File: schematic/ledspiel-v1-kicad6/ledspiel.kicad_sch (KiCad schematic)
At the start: 133 parts, among them J1 Conn_Battery, J3 USART Debug, J4 Micro_SD_Card, J5 USB_B_Micro, J50 Conn_01x16_Male, Q1 BSS138, Q10 BSS138, Q11 BSS138, Q12 BSS138, Q13 BSS138, Q14 BSS138, Q40 IRLML6402, Q60 SFH300-3/4, U1 STM32F405RGTx, U2 USBLC6-2SC6, U3 MCP1640CH, U4 LP38693MP-3.3, U6 TSOP312xx, Y1 8MHz, Y2 32768Hz

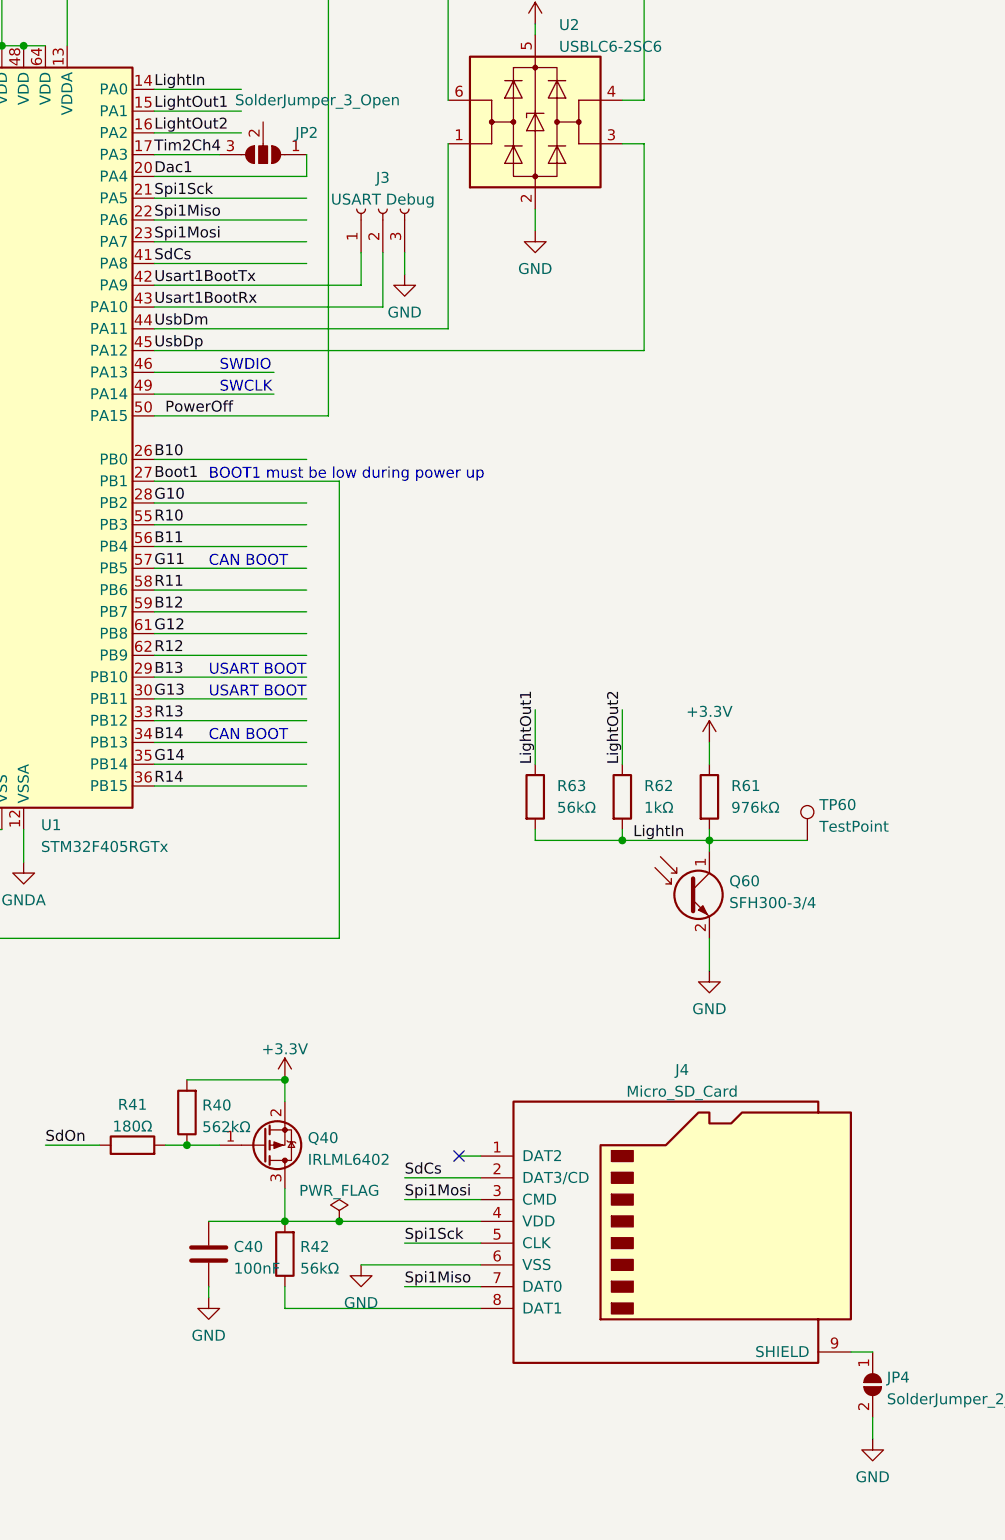
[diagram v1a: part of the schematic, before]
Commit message: WIP: Add LM
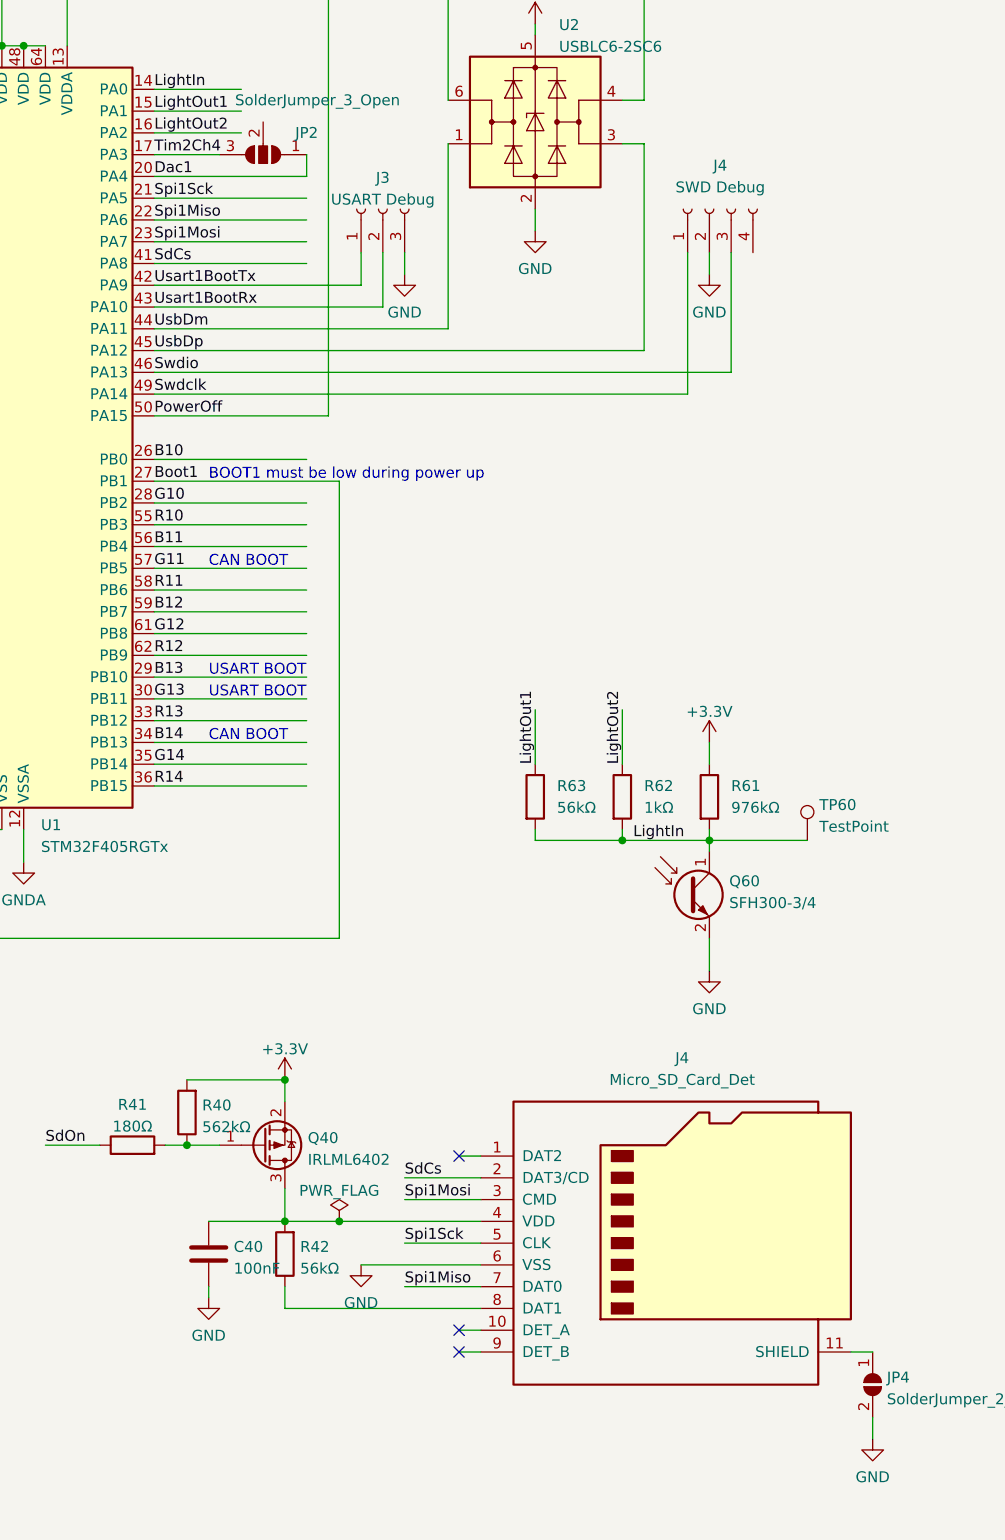
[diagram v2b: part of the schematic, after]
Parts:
- removed J4: Micro_SD_Card, symbol Connector:Micro_SD_Card
- added J4: SWD Debug, symbol Connector:Conn_01x04_Female
- added J4: Micro_SD_Card_Det, symbol Connector:Micro_SD_Card_Det
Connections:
- net GND: now also J4.2 (Pin_2), J4.6 (VSS)
- net SdCs: now also J4.2 (DAT3/CD)
- net Spi1Miso: now also J4.7 (DAT0)
- net Spi1Mosi: now also J4.3 (CMD)
- net Spi1Sck: now also J4.5 (CLK)
- net Swdio: now reaches U1.46 (PA13)
- net Swdio: now also J4.3 (Pin_3)
- net Swdclk: now reaches U1.49 (PA14)
- net Swdclk: now also J4.1 (Pin_1)
- net at R42.1: now also J4.8 (DAT1)
- net at C40.1, Q40.3 (D), R42.2: now also J4.4 (VDD)
- net at JP4.1 (A): now also J4.11 (SHIELD)
- no-connect marks 2 -> 4
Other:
- note removed: "SWCLK"
- note removed: "SWDIO"
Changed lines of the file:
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@@
   (junction (at 67.31 55.88) (diameter 0) (color 0 0 0 0)
   )
+  (no_connect (at 157.48 250.19))
   (no_connect (at 173.99 78.74))
   (no_connect (at 157.48 229.87))
+  (no_connect (at 157.48 252.73))
   (wire (pts (xy 299.72 77.47) (xy 299.72 102.87))
     (stroke (width 0) (type default) (color 0 0 0 0))
@@
     (stroke (width 0) (type default) (color 0 0 0 0))
   )
-  (wire (pts (xy 121.92 138.43) (xy 135.89 138.43))
+  (wire (pts (xy 121.92 138.43) (xy 189.23 138.43))
     (stroke (width 0) (type default) (color 0 0 0 0))
   )
@@
     (stroke (width 0) (type default) (color 0 0 0 0))
   )
+  (wire (pts (xy 189.23 124.46) (xy 189.23 138.43))
+    (stroke (width 0) (type default) (color 0 0 0 0))
+  )
   (wire (pts (xy 297.18 107.95) (xy 297.18 133.35))
     (stroke (width 0) (type default) (color 0 0 0 0))
@@
     (stroke (width 0) (type default) (color 0 0 0 0))
   )
+  (wire (pts (xy 184.15 124.46) (xy 184.15 140.97))
+    (stroke (width 0) (type default) (color 0 0 0 0))
+  )
   (wire (pts (xy 121.92 184.15) (xy 139.7 184.15))
     (stroke (width 0) (type default) (color 0 0 0 0))
@@
     (stroke (width 0) (type default) (color 0 0 0 0))
   )
+  (wire (pts (xy 186.69 124.46) (xy 186.69 127))
+    (stroke (width 0) (type default) (color 0 0 0 0))
+  )
   (wire (pts (xy 67.31 44.45) (xy 67.31 45.72))
     (stroke (width 0) (type default) (color 0 0 0 0))
@@
     (stroke (width 0) (type default) (color 0 0 0 0))
   )
-  (wire (pts (xy 121.92 140.97) (xy 135.89 140.97))
+  (wire (pts (xy 121.92 140.97) (xy 184.15 140.97))
     (stroke (width 0) (type default) (color 0 0 0 0))
   )
@@
     (stroke (width 0) (type default) (color 0 0 0 0))
   )
+  (wire (pts (xy 157.48 252.73) (xy 160.02 252.73))
+    (stroke (width 0) (type default) (color 0 0 0 0))
+  )
   (wire (pts (xy 290.83 52.07) (xy 299.72 52.07))
     (stroke (width 0) (type default) (color 0 0 0 0))
@@
     (stroke (width 0) (type default) (color 0 0 0 0))
   )
+  (wire (pts (xy 157.48 250.19) (xy 160.02 250.19))
+    (stroke (width 0) (type default) (color 0 0 0 0))
+  )
   (wire (pts (xy 151.13 86.36) (xy 151.13 83.82))
     (stroke (width 0) (type default) (color 0 0 0 0))
@@
     (effects (font (size 1.27 1.27)) (justify left bottom))
   )
-  (text "SWCLK" (at 129.54 140.97 0)
-    (effects (font (size 1.27 1.27)) (justify left bottom))
-  )
-  (text "SWDIO" (at 129.54 138.43 0)
-    (effects (font (size 1.27 1.27)) (justify left bottom))
-  )
   (label "Line5" (at 241.3 149.86 0)
     (effects (font (size 1.27 1.27)) (justify left bottom))
@@
     (effects (font (size 1.27 1.27)) (justify left bottom))
   )
+  (label "Swdio" (at 121.92 138.43 0)
+    (effects (font (size 1.27 1.27)) (justify left bottom))
+  )
+  (label "Swdclk" (at 121.92 140.97 0)
+    (effects (font (size 1.27 1.27)) (justify left bottom))
+  )
   (label "Line5" (at 81.28 158.75 0)
     (effects (font (size 1.27 1.27)) (justify left bottom))
@@
     (effects (font (size 1.27 1.27)) (justify left bottom))
   )
-  (label "PowerOff" (at 123.19 143.51 0)
+  (label "PowerOff" (at 121.92 143.51 0)
     (effects (font (size 1.27 1.27)) (justify left bottom))
   )
@@
     (pin "1")
   )
+  (symbol (lib_id "Connector:Conn_01x04_Female") (at 186.69 119.38 90) (unit 1)
+    (in_bom yes) (on_board yes) (fields_autoplaced)
+    (property "Reference" "J4" (id 0) (at 187.96 114.3 90))
+    (property "Value" "SWD Debug" (id 1) (at 187.96 116.84 90))
+    (property "Footprint" "" (id 2) (at 186.69 119.38 0)
+      (effects (font (size 1.27 1.27)) hide)
+    )
+    (property "Datasheet" "~" (id 3) (at 186.69 119.38 0)
+      (effects (font (size 1.27 1.27)) hide)
+    )
+    (pin "1")
+    (pin "2")
+    (pin "3")
+    (pin "4")
+  )
   (symbol (lib_id "power:GND") (at 146.05 242.57 0) (unit 1)
     (in_bom yes) (on_board yes) (fields_autoplaced)
@@
     (pin "3")
   )
-  (symbol (lib_id "Connector:Micro_SD_Card") (at 182.88 237.49 0) (unit 1)
-    (in_bom yes) (on_board yes) (fields_autoplaced)
-    (property "Reference" "J4" (id 0) (at 183.515 219.8202 0))
-    (property "Value" "Micro_SD_Card" (id 1) (at 183.515 222.3571 0))
-    (property "Footprint" "" (id 2) (at 212.09 229.87 0)
-      (effects (font (size 1.27 1.27)) hide)
-    )
-    (property "Datasheet" "http://katalog.we-online.de/em/datasheet/693072010801.pdf" (id 3) (at 182.88 237.49 0)
-      (effects (font (size 1.27 1.27)) hide)
-    )
-    (pin "1")
-    (pin "2")
-    (pin "3")
-    (pin "4")
-    (pin "5")
-    (pin "6")
-    (pin "7")
-    (pin "8")
-    (pin "9")
-  )
   (symbol (lib_id "Device:LED_RKGB") (at 285.75 133.35 0) (unit 1)
     (in_bom yes) (on_board yes) (fields_autoplaced)
@@
     (pin "1")
   )
+  (symbol (lib_id "Connector:Micro_SD_Card_Det") (at 182.88 240.03 0) (unit 1)
+    (in_bom yes) (on_board yes) (fields_autoplaced)
+    (property "Reference" "J4" (id 0) (at 183.515 218.44 0))
+    (property "Value" "Micro_SD_Card_Det" (id 1) (at 183.515 220.98 0))
+    (property "Footprint" "" (id 2) (at 234.95 222.25 0)
+      (effects (font (size 1.27 1.27)) hide)
+    )
+    (property "Datasheet" "https://www.hirose.com/product/en/download_file/key_name/DM3/category/Catalog/doc_file_id/49662/?file_category_id=4&item_id=195&is_series=1" (id 3) (at 182.88 237.49 0)
+      (effects (font (size 1.27 1.27)) hide)
+    )
+    (pin "1")
+    (pin "10")
+    (pin "11")
+    (pin "2")
+    (pin "3")
+    (pin "4")
+    (pin "5")
+    (pin "6")
+    (pin "7")
+    (pin "8")
+    (pin "9")
+  )
   (symbol (lib_id "power:GND") (at 265.43 132.08 0) (unit 1)
     (in_bom yes) (on_board yes)
@@
     (pin "2")
   )
+  (symbol (lib_id "power:GND") (at 186.69 127 0) (unit 1)
+    (in_bom yes) (on_board yes) (fields_autoplaced)
+    (property "Reference" "#PWR?" (id 0) (at 186.69 133.35 0)
+      (effects (font (size 1.27 1.27)) hide)
+    )
+    (property "Value" "GND" (id 1) (at 186.69 131.4434 0))
+    (property "Footprint" "" (id 2) (at 186.69 127 0)
+      (effects (font (size 1.27 1.27)) hide)
+    )
+    (property "Datasheet" "" (id 3) (at 186.69 127 0)
+      (effects (font (size 1.27 1.27)) hide)
+    )
+    (pin "1")
+  )
   (symbol (lib_id "Power_Protection:USBLC6-2SC6") (at 166.37 109.22 0) (unit 1)
     (in_bom yes) (on_board yes) (fields_autoplaced)
@@
       (reference "#PWR0145") (unit 1) (value "GND") (footprint "")
     )
+    (path "/cdbf996f-f703-47a9-b942-793d49c769fa"
+      (reference "#PWR?") (unit 1) (value "GND") (footprint "")
+    )
     (path "/315ec405-f84d-41f5-b6ee-59d298dca57a"
       (reference "C1") (unit 1) (value "10µF") (footprint "")
@@
       (reference "J3") (unit 1) (value "USART Debug") (footprint "")
     )
-    (path "/b10fb92a-abe2-4cf8-8650-b7aa5f625383"
-      (reference "J4") (unit 1) (value "Micro_SD_Card") (footprint "")
+    (path "/70c16904-7537-4c0a-b3a3-fa64963865fb"
+      (reference "J4") (unit 1) (value "SWD Debug") (footprint "")
+    )
+    (path "/bb0243ca-9a80-4200-9d6a-0017ad774b60"
+      (reference "J4") (unit 1) (value "Micro_SD_Card_Det") (footprint "Connector_Card:microSD_HC_Hirose_DM3D-SF")
     )
     (path "/145f17d5-7130-4b50-b488-eb854900bf1f"

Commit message: WIP
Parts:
- removed JP4: SolderJumper_2_Open, symbol Jumper:SolderJumper_2_Open
- added C100: 100nF, symbol Device:C
- added C101, C102: 2.2µF, symbol Device:C
- added C103: 18nF, symbol Device:C
- added JP100: SolderJumper_3_Open, symbol Jumper:SolderJumper_3_Open
- added R100: 330kΩ, symbol Device:R
- added R101: 56kΩ, symbol Device:R
- added R102: 200Ω, symbol Device:R
- added R73, R74, R75: 47Ω, symbol Device:R
- added RV100: 25kΩ, symbol Device:R_Potentiometer
- added U100: LM4861, Package_SO:SOIC-8-N7_3.9x4.9mm_P1.27mm, symbol malteLib2025:LM4861
- C70: renamed from C40; value 100nF -> 2.2µF
- J70: renamed from J4; footprint (none) -> Connector_Card:microSD_HC_Hirose_DM3D-SF
- R50, R51, R52, R53, R54, R55, R56, R57, R60: value 180Ω -> 200Ω
- R70: renamed from R41; value 180Ω -> 200Ω
- R71: renamed from R40; value 562kΩ -> 330kΩ
- R9: value 10kΩ -> 100kΩ
- renumbered JP2 to JP101, LS1 to LS100, Q40 to Q70, R42 to R72, U6 to U60
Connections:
- net Dac1: now also JP101.3 (B), JP100.3 (B); no longer JP101.1 (A)
- net GND: now also J70.11 (SHIELD)
- net GNDA: now also C100.2, C101.2, C103.2, U100.7 (GND)
- net Spi1Miso: now also R75.1; no longer J70.7 (DAT0)
- net Spi1Mosi: now also R73.1; no longer J70.3 (CMD)
- net Spi1Sck: now also R74.1; no longer J70.5 (CLK)
- net Tim2Ch4: now also JP101.1 (A), JP100.1 (A); no longer JP101.3 (B)
- net VDDA: now also C100.1, R100.2, U100.6 (VDD)
- net at R9.1, U1.7 (NRST): now also J4.4 (Pin_4)
- net at JP101.2 (C): now also R102.1
- net at LS100.1: now also RV100.2, U100.5 (Vo1)
- net at LS100.2: now also U100.8 (Vo2)
- new net: JP100.2 (C), R100.1, U100.1 (SHDN)
- new net: C101.1, U100.2 (BYPASS), U100.3 (IN+)
- new net: R101.2, U100.4 (IN-)
- new net: J70.5 (CLK), R74.2
- new net: C102.2, R101.1, RV100.3
- new net: C102.1, C103.1, R102.2
- new net: J70.3 (CMD), R73.2
- new net: J70.7 (DAT0), R75.2
- no-connect marks 4 -> 5
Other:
- note added: "C103 only if PWM is used"
- note added: "Namings: 0...9: STM32 + I/O + USB 10...59: LED Matrix 60...69: Brightness and IR input 70...79: SD card 80...99: Power supply 100...109: Sound"
- note added: "One pin of the STM provides audio data the other controls the shutdown"
- note added: "maximum gain: 0.89"
- moved on the sheet: C10, C11, C12, C13, C14, C15, C16, C60, C7, C70, C8, C9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
